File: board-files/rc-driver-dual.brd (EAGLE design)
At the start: 31 x 17.5 mm, 18 parts

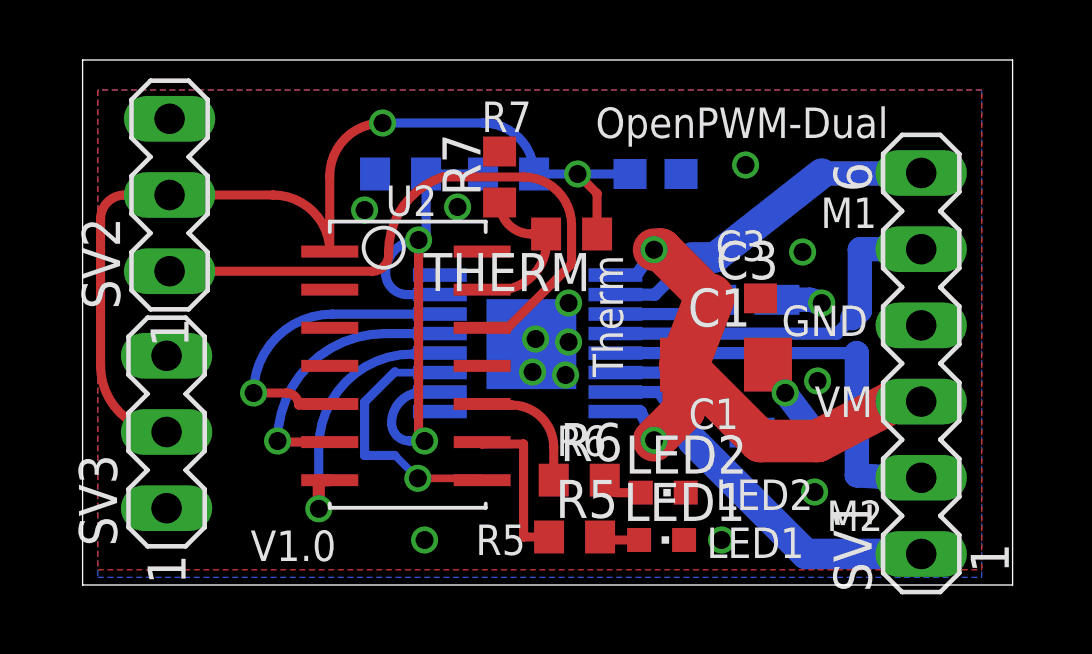
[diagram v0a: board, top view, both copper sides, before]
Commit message: add drunken spriral
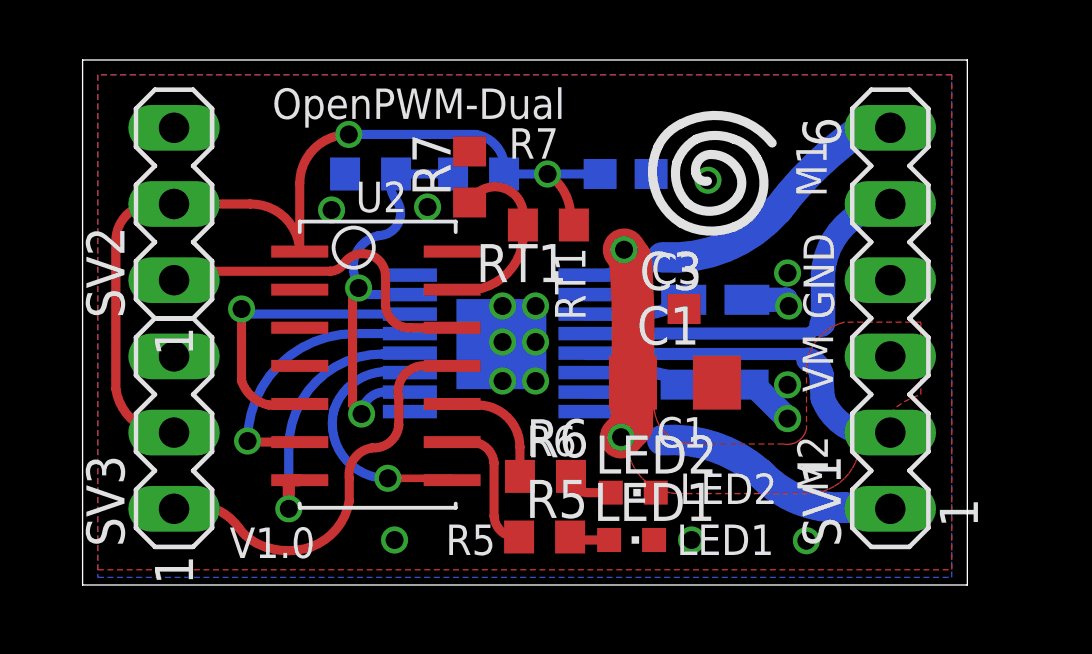
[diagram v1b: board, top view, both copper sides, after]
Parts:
- removed THERM: (no value), resistor:R0603
- added RT1: (no value), resistor:R0603
- moved R1 2.80 mm to (21.1, 6.68)
- moved C3 2.57 mm to (19.2, 9.20)
- moved SV1 1.82 mm to (26.9, 8.89)
- moved C1 1.80 mm to (19.7, 6.74)
- moved R6 1.13 mm to (15.4, 3.62)
- moved C2 1.00 mm to (18.1, 13.7)
- moved LED1 1.00 mm to (18.3, 1.50)
- moved LED2 1.00 mm to (18.4, 3.08)
- moved R2 1.00 mm to (21.1, 9.51)
- moved R3 1.00 mm to (13.2, 13.7)
- moved R4 1.00 mm to (9.60, 13.7)
- moved R7 1.00 mm to (12.9, 13.6)
- moved U$1 1.00 mm to (9.78, 8.57)
- moved U$2 1.00 mm to (14.2, 7.85)
- moved R5 1.00 mm to (15.4, 1.60)
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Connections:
- removed net N$24: U$1.P$4
- removed net N$26: U$1.P$3
- removed net N$27: U$1.P$2
- removed net N$5: U$1.P$11
- net +5V: now also RT1.1; no longer THERM.1
- net PWM2: now also U$1.P$11
- net T-OUT: now also RT1.2; no longer THERM.2
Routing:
- net PWM2: track 0.00 -> 13.2 mm
- net VM: track 21.2 -> 9.96 mm
- net PWM1: track 20.8 -> 10.8 mm
- net VREF: track 18.5 -> 14.1 mm
- net MOTOR2-1: track 14.8 -> 11.6 mm
- net +5V: track 33.0 -> 30.2 mm
- net N$1: track 5.46 -> 3.31 mm
- net MOTOR2-2: track 12.6 -> 11.3 mm
- net LED: track 5.40 -> 4.58 mm
- net OUTPUT3: track 8.98 -> 8.17 mm
- net GND: track 3.17 -> 3.37 mm, vias 15 -> 16
- added copper zone on layer 1, net VM
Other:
- board size 31 x 17.5 mm -> 29.5 x 17.5 mm
- board text added: "RT1"
- board text removed: "Therm"
